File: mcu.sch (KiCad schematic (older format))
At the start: 18 parts, among them J501 JTAG, J502 Serial / Bootloader, SW501 EVQQ2, SW502 EVQQ2, U501 STM32F405RGTx, Y501 8MHz

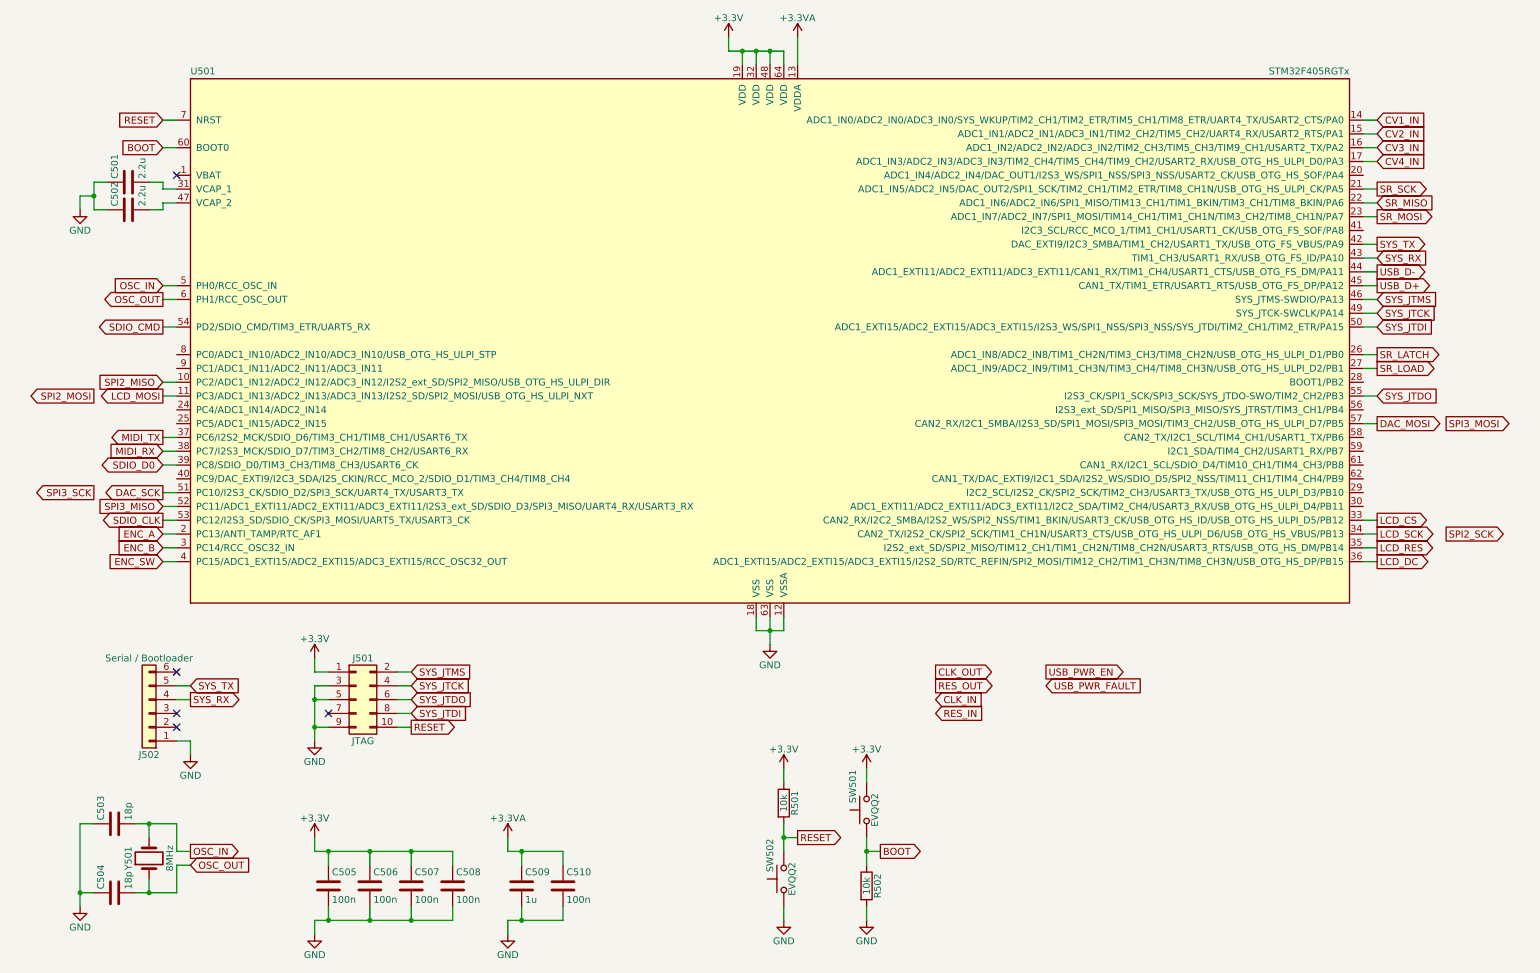
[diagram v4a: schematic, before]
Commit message: only ground plane left
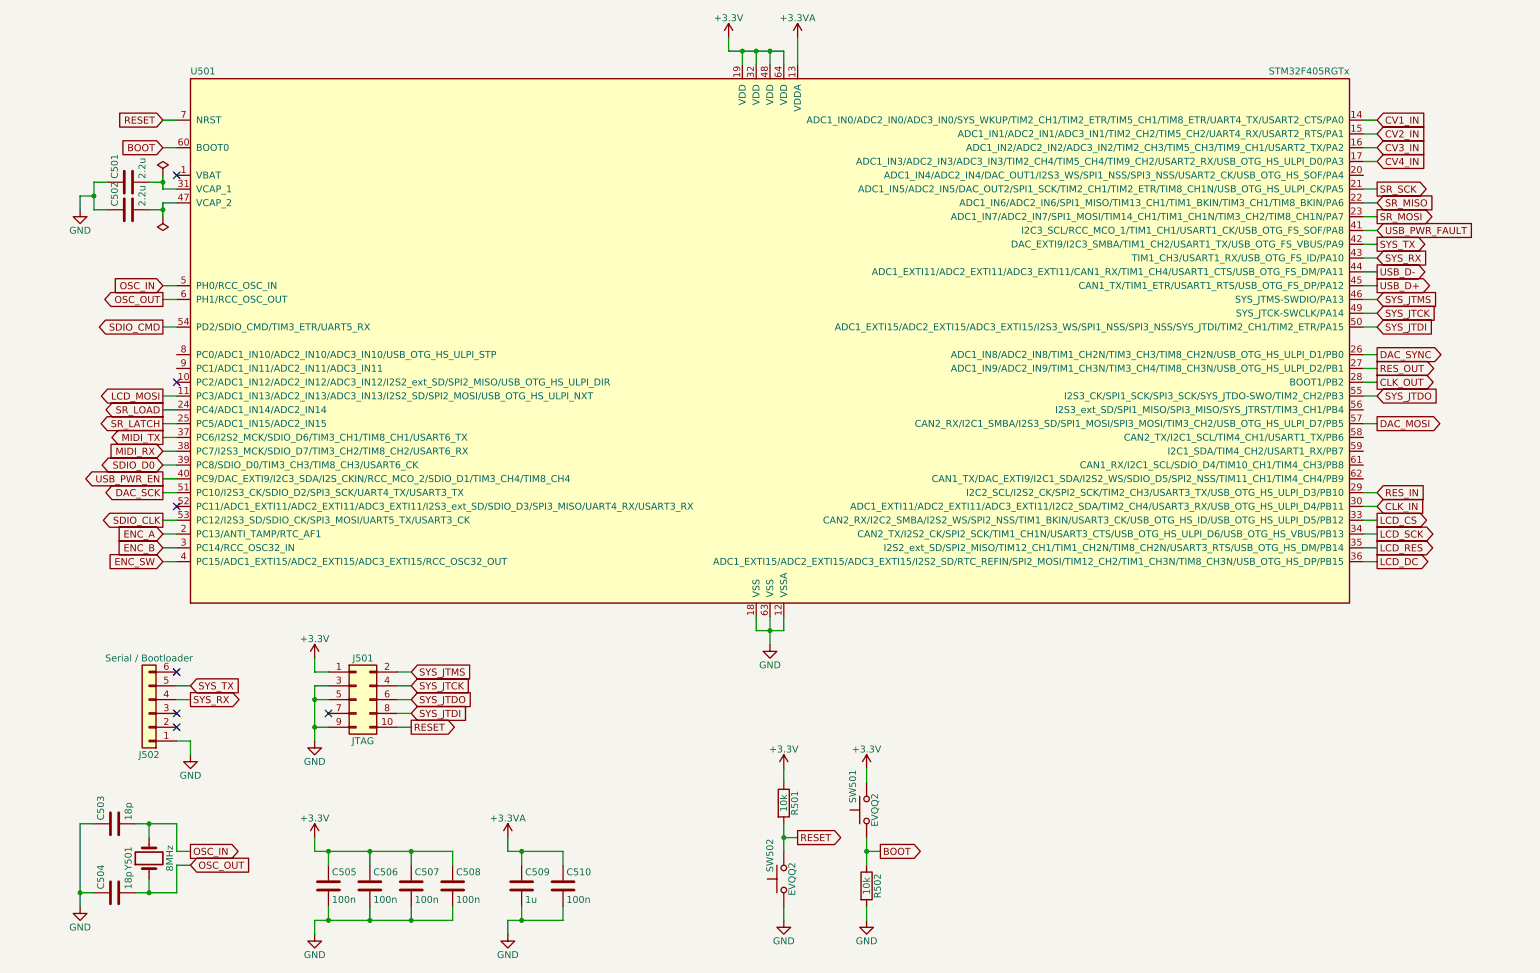
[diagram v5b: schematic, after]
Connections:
- net CLK_IN: now also U501.30 (ADC1_EXTI11/ADC2_EXTI11/ADC3_EXTI11/I2C2_SDA/TIM2_CH4/USART3_RX/USB_OTG_HS_ULPI_D4/PB11)
- net CLK_OUT: now also U501.28 (BOOT1/PB2)
- net RES_IN: now also U501.29 (I2C2_SCL/I2S2_CK/SPI2_SCK/TIM2_CH3/USART3_TX/USB_OTG_HS_ULPI_D3/PB10)
- net RES_OUT: now also U501.27 (ADC1_IN9/ADC2_IN9/TIM1_CH3N/TIM3_CH4/TIM8_CH3N/USB_OTG_HS_ULPI_D2/PB1)
- net SR_LATCH: now also U501.25 (PC5/ADC1_IN15/ADC2_IN15); no longer U501.26 (ADC1_IN8/ADC2_IN8/TIM1_CH2N/TIM3_CH3/TIM8_CH2N/USB_OTG_HS_ULPI_D1/PB0)
- net SR_LOAD: now also U501.24 (PC4/ADC1_IN14/ADC2_IN14); no longer U501.27 (ADC1_IN9/ADC2_IN9/TIM1_CH3N/TIM3_CH4/TIM8_CH3N/USB_OTG_HS_ULPI_D2/PB1)
- net USB_PWR_EN: now also U501.40 (PC9/DAC_EXTI9/I2C3_SDA/I2S_CKIN/RCC_MCO_2/SDIO_D1/TIM3_CH4/TIM8_CH4)
- net USB_PWR_FAULT: now also U501.41 (I2C3_SCL/RCC_MCO_1/TIM1_CH1/USART1_CK/USB_OTG_FS_SOF/PA8)
- net SPI2_MISO: no longer names the net of U501.10 (PC2/ADC1_IN12/ADC2_IN12/ADC3_IN12/I2S2_ext_SD/SPI2_MISO/USB_OTG_HS_ULPI_DIR)
- net SPI3_MISO: no longer names the net of U501.52 (PC11/ADC1_EXTI11/ADC2_EXTI11/ADC3_EXTI11/I2S3_ext_SD/SDIO_D3/SPI3_MISO/UART4_RX/USART3_RX)
- new net DAC_SYNC: U501.26 (ADC1_IN8/ADC2_IN8/TIM1_CH2N/TIM3_CH3/TIM8_CH2N/USB_OTG_HS_ULPI_D1/PB0)
- no-connect marks 5 -> 7
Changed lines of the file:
@@
 $EndComp
 $Comp
-L GND #PWR507
+L GND #PWR050
 U 1 1 59DB9615
 P 1600 6200
-F 0 "#PWR507" H 1600 5950 50  0001 C CNN
+F 0 "#PWR050" H 1600 5950 50  0001 C CNN
 F 1 "GND" H 1600 6050 50  0000 C CNN
 F 2 "" H 1600 6200 50  0001 C CNN
@@
 $EndComp
 $Comp
-L +3.3V #PWR505
+L +3.3V #PWR051
 U 1 1 59DB9CCC
 P 2500 5500
-F 0 "#PWR505" H 2500 5350 50  0001 C CNN
+F 0 "#PWR051" H 2500 5350 50  0001 C CNN
 F 1 "+3.3V" H 2500 5640 50  0000 C CNN
 F 2 "" H 2500 5500 50  0001 C CNN
@@
 $EndComp
 $Comp
-L GND #PWR506
+L GND #PWR052
 U 1 1 59DB9CF4
 P 2500 6100
-F 0 "#PWR506" H 2500 5850 50  0001 C CNN
+F 0 "#PWR052" H 2500 5850 50  0001 C CNN
 F 1 "GND" H 2500 5950 50  0000 C CNN
 F 2 "" H 2500 6100 50  0001 C CNN
@@
 $EndComp
 $Comp
-L +3.3V #PWR501
+L +3.3V #PWR053
 U 1 1 59DB9EAC
 P 5500 1000
-F 0 "#PWR501" H 5500 850 50  0001 C CNN
+F 0 "#PWR053" H 5500 850 50  0001 C CNN
 F 1 "+3.3V" H 5500 1140 50  0000 C CNN
 F 2 "" H 5500 1000 50  0001 C CNN
@@
 $EndComp
 $Comp
-L +3.3VA #PWR502
+L +3.3VA #PWR054
 U 1 1 59DB9EE7
 P 6000 1000
-F 0 "#PWR502" H 6000 850 50  0001 C CNN
+F 0 "#PWR054" H 6000 850 50  0001 C CNN
 F 1 "+3.3VA" H 6000 1140 50  0000 C CNN
 F 2 "" H 6000 1000 50  0001 C CNN
@@
 $EndComp
 $Comp
-L GND #PWR504
+L GND #PWR055
 U 1 1 59DB9FE7
 P 5800 5400
-F 0 "#PWR504" H 5800 5150 50  0001 C CNN
+F 0 "#PWR055" H 5800 5150 50  0001 C CNN
 F 1 "GND" H 5800 5250 50  0000 C CNN
 F 2 "" H 5800 5400 50  0001 C CNN
@@
 $EndComp
 $Comp
-L GND #PWR512
+L GND #PWR056
 U 1 1 59DBA437
 P 800 7300
-F 0 "#PWR512" H 800 7050 50  0001 C CNN
+F 0 "#PWR056" H 800 7050 50  0001 C CNN
 F 1 "GND" H 800 7150 50  0000 C CNN
 F 2 "" H 800 7300 50  0001 C CNN
@@
 $EndComp
 $Comp
-L GND #PWR503
+L GND #PWR057
 U 1 1 59DBB736
 P 800 2250
-F 0 "#PWR503" H 800 2000 50  0001 C CNN
+F 0 "#PWR057" H 800 2000 50  0001 C CNN
 F 1 "GND" H 800 2100 50  0000 C CNN
 F 2 "" H 800 2250 50  0001 C CNN
@@
 $EndComp
 $Comp
-L +3.3V #PWR508
+L +3.3V #PWR058
 U 1 1 59DD49A9
 P 5900 6300
-F 0 "#PWR508" H 5900 6150 50  0001 C CNN
+F 0 "#PWR058" H 5900 6150 50  0001 C CNN
 F 1 "+3.3V" H 5900 6440 50  0000 C CNN
 F 2 "" H 5900 6300 50  0001 C CNN
@@
 $EndComp
 $Comp
-L +3.3V #PWR509
+L +3.3V #PWR059
 U 1 1 59DD49E1
 P 6500 6300
-F 0 "#PWR509" H 6500 6150 50  0001 C CNN
+F 0 "#PWR059" H 6500 6150 50  0001 C CNN
 F 1 "+3.3V" H 6500 6440 50  0000 C CNN
 F 2 "" H 6500 6300 50  0001 C CNN
@@
 $EndComp
 $Comp
-L GND #PWR513
+L GND #PWR060
 U 1 1 59DD4A83
 P 5900 7400
-F 0 "#PWR513" H 5900 7150 50  0001 C CNN
+F 0 "#PWR060" H 5900 7150 50  0001 C CNN
 F 1 "GND" H 5900 7250 50  0000 C CNN
 F 2 "" H 5900 7400 50  0001 C CNN
@@
 $EndComp
 $Comp
-L GND #PWR514
+L GND #PWR061
 U 1 1 59DD4ABB
 P 6500 7400
-F 0 "#PWR514" H 6500 7150 50  0001 C CNN
+F 0 "#PWR061" H 6500 7150 50  0001 C CNN
 F 1 "GND" H 6500 7250 50  0000 C CNN
 F 2 "" H 6500 7400 50  0001 C CNN
@@
 $EndComp
 $Comp
-L +3.3V #PWR510
+L +3.3V #PWR062
 U 1 1 59E34B90
 P 2500 6800
-F 0 "#PWR510" H 2500 6650 50  0001 C CNN
+F 0 "#PWR062" H 2500 6650 50  0001 C CNN
 F 1 "+3.3V" H 2500 6940 50  0000 C CNN
 F 2 "" H 2500 6800 50  0001 C CNN
@@
 $EndComp
 $Comp
-L GND #PWR515
+L GND #PWR063
 U 1 1 59E34BD4
 P 2500 7500
-F 0 "#PWR515" H 2500 7250 50  0001 C CNN
+F 0 "#PWR063" H 2500 7250 50  0001 C CNN
 F 1 "GND" H 2500 7350 50  0000 C CNN
 F 2 "" H 2500 7500 50  0001 C CNN
@@
 $EndComp
 $Comp
-L +3.3VA #PWR511
+L +3.3VA #PWR064
 U 1 1 59E35078
 P 3900 6800
-F 0 "#PWR511" H 3900 6650 50  0001 C CNN
+F 0 "#PWR064" H 3900 6650 50  0001 C CNN
 F 1 "+3.3VA" H 3900 6940 50  0000 C CNN
 F 2 "" H 3900 6800 50  0001 C CNN
@@
 $EndComp
 $Comp
-L GND #PWR516
+L GND #PWR065
 U 1 1 59E350BC
 P 3900 7500
-F 0 "#PWR516" H 3900 7250 50  0001 C CNN
+F 0 "#PWR065" H 3900 7250 50  0001 C CNN
 F 1 "GND" H 3900 7350 50  0000 C CNN
 F 2 "" H 3900 7500 50  0001 C CNN
@@
 Text GLabel 1400 4800 0    51   Input ~ 0
 ENC_SW
-Text GLabel 1400 3500 0    51   Input ~ 0
-SPI2_MISO
-Text GLabel 900  3600 0    51   Output ~ 0
-SPI2_MOSI
-Text GLabel 10700 4600 2    51   Output ~ 0
-SPI2_SCK
-Text GLabel 10700 3800 2    51   Output ~ 0
-SPI3_MOSI
-Text GLabel 900  4300 0    51   Output ~ 0
-SPI3_SCK
-Text GLabel 1400 4400 0    51   Input ~ 0
-SPI3_MISO
 Text GLabel 10200 1600 2    51   Input ~ 0
 CV1_IN
@@
 Text GLabel 10200 1900 2    51   Input ~ 0
 CV4_IN
-Text GLabel 7000 5600 2    51   Output ~ 0
+Text GLabel 10200 3500 2    51   Output ~ 0
 CLK_OUT
-Text GLabel 7000 5700 2    51   Output ~ 0
+Text GLabel 10200 3400 2    51   Output ~ 0
 RES_OUT
-Text GLabel 7000 5800 2    51   Input ~ 0
+Text GLabel 10200 4400 2    51   Input ~ 0
 CLK_IN
-Text GLabel 7000 5900 2    51   Input ~ 0
+Text GLabel 10200 4300 2    51   Input ~ 0
 RES_IN
 Text GLabel 10200 2300 2    51   Output ~ 0
@@
 Text GLabel 10200 2100 2    51   Output ~ 0
 SR_SCK
-Text GLabel 10200 3300 2    51   Output ~ 0
+Text GLabel 1400 3800 0    51   Output ~ 0
 SR_LATCH
-Text GLabel 10200 3400 2    51   Output ~ 0
+Text GLabel 1400 3700 0    51   Output ~ 0
 SR_LOAD
 Text GLabel 10200 3800 2    51   Output ~ 0
@@
 Text GLabel 1400 4300 0    51   Output ~ 0
 DAC_SCK
-Text GLabel 7800 5600 2    51   Output ~ 0
+Text GLabel 1400 4200 0    51   Output ~ 0
 USB_PWR_EN
-Text GLabel 7800 5700 2    51   Input ~ 0
+Text GLabel 10200 2400 2    51   Input ~ 0
 USB_PWR_FAULT
 Text GLabel 10200 2700 2    51   Output ~ 0
@@
 	10100 3600 10200 3600
 Wire Wire Line
-	1500 2100 1400 2100
-Wire Wire Line
-	1400 2100 1400 2050
+	1400 2100 1500 2100
+Wire Wire Line
+	1400 2000 1400 2100
 Wire Wire Line
 	1400 2050 1300 2050
@@
 	1500 2200 1400 2200
 Wire Wire Line
-	1400 2200 1400 2250
+	1400 2200 1400 2300
 Wire Wire Line
 	1400 2250 1300 2250
@@
 	10100 2300 10200 2300
 Wire Wire Line
-	1500 3500 1400 3500
-Wire Wire Line
 	1500 3600 1400 3600
 Wire Wire Line
@@
 Wire Wire Line
 	1400 4300 1500 4300
-Wire Wire Line
-	1400 4400 1500 4400
 Wire Wire Line
 	10100 1600 10200 1600
@@
 NoConn ~ 2600 5900
 NoConn ~ 1500 2000
+Text GLabel 10200 3300 2    51   Output ~ 0
+DAC_SYNC
+Wire Wire Line
+	1400 3700 1500 3700
+Wire Wire Line
+	1400 3800 1500 3800
+Wire Wire Line
+	10100 3500 10200 3500
+Wire Wire Line
+	10100 4300 10200 4300
+NoConn ~ 1500 3500
+NoConn ~ 1500 4400
+Wire Wire Line
+	10200 4400 10100 4400
+Wire Wire Line
+	10200 2400 10100 2400
+Wire Wire Line
+	1400 4200 1500 4200
+$Comp
+L PWR_FLAG #FLG066
+U 1 1 59F48B1D
+P 1400 2300
+F 0 "#FLG066" H 1400 2375 50  0001 C CNN
+F 1 "PWR_FLAG" H 1400 2450 50  0001 C CNN
+F 2 "" H 1400 2300 50  0001 C CNN
+F 3 "" H 1400 2300 50  0001 C CNN
+	1    1400 2300
+	-1   0    0    1
+$EndComp
+Connection ~ 1400 2250
+$Comp
+L PWR_FLAG #FLG067
+U 1 1 59F48C86
+P 1400 2000
+F 0 "#FLG067" H 1400 2075 50  0001 C CNN
+F 1 "PWR_FLAG" H 1400 2150 50  0001 C CNN
+F 2 "" H 1400 2000 50  0001 C CNN
+F 3 "" H 1400 2000 50  0001 C CNN
+	1    1400 2000
+	1    0    0    -1
+$EndComp
+Connection ~ 1400 2050
 $EndSCHEMATC
